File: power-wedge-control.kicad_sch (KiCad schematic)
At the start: 58 parts, among them J1 Conn_01x02, J2 Conn_01x03, J3 Conn_01x02, J4 Conn_01x03, J5 Conn_01x03, J6 Conn_01x06_Female, J7 Conn_01x04_Female, J8 Conn_01x03, J9 MicroSD_Hirose_DM3D-SF, Q1 MMBT3904L, Q2 DMP3099L, Q3 MMBT3904L, Q4 DMP3099L, Q5 MMBT3904L, Q6 MMBT3904L, U1 LM7805_TO220, U3 TLV70233DBV, U4 4050

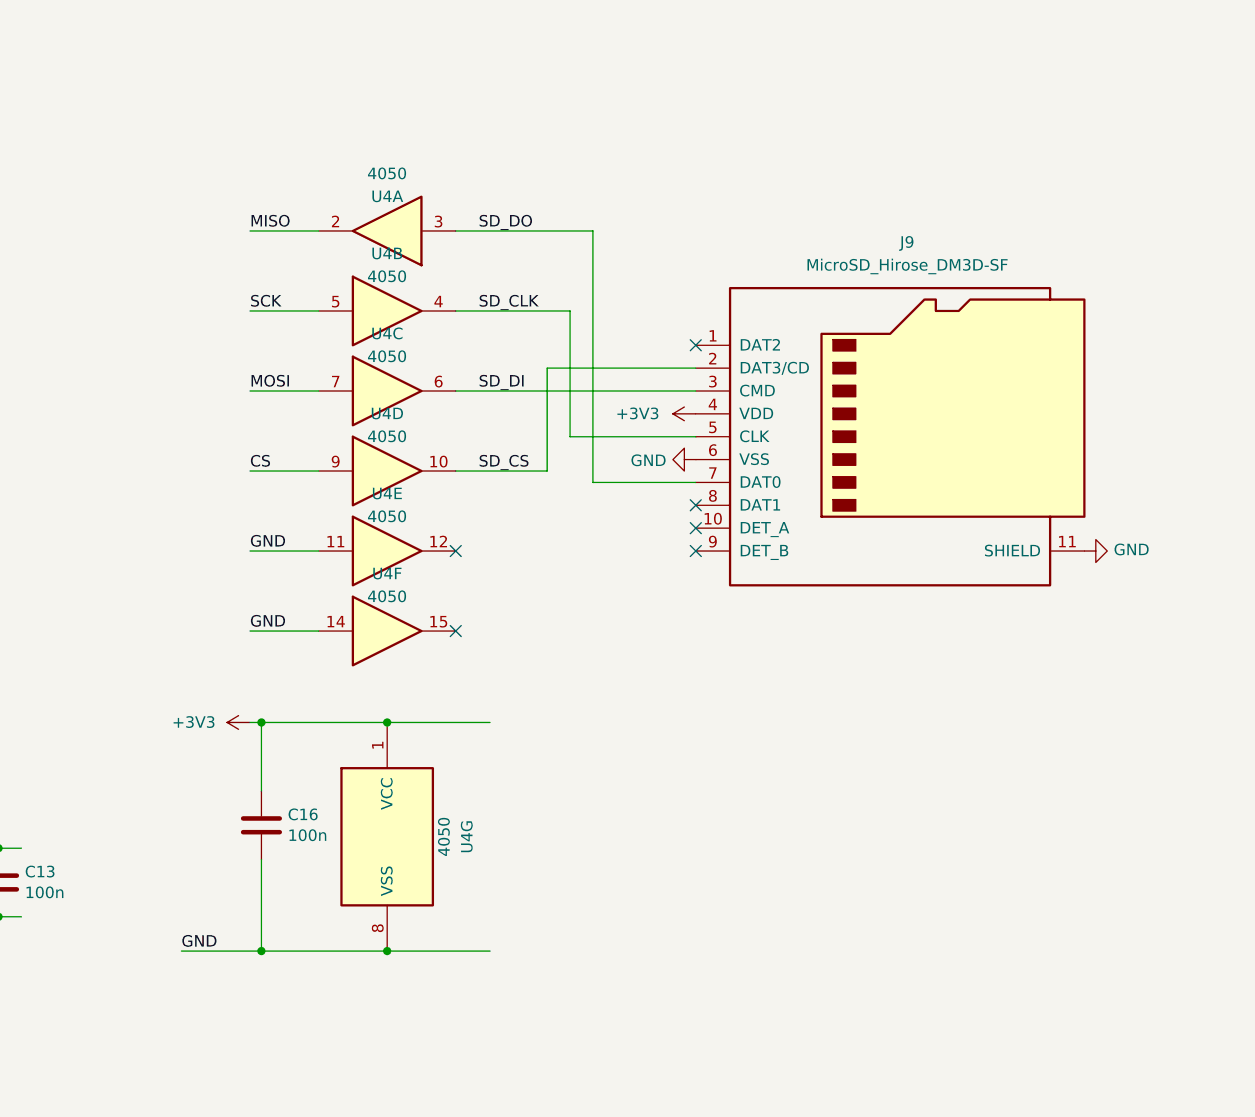
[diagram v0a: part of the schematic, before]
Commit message: Switch to NC7WZ17P6X buffers for level shifting to SD card.
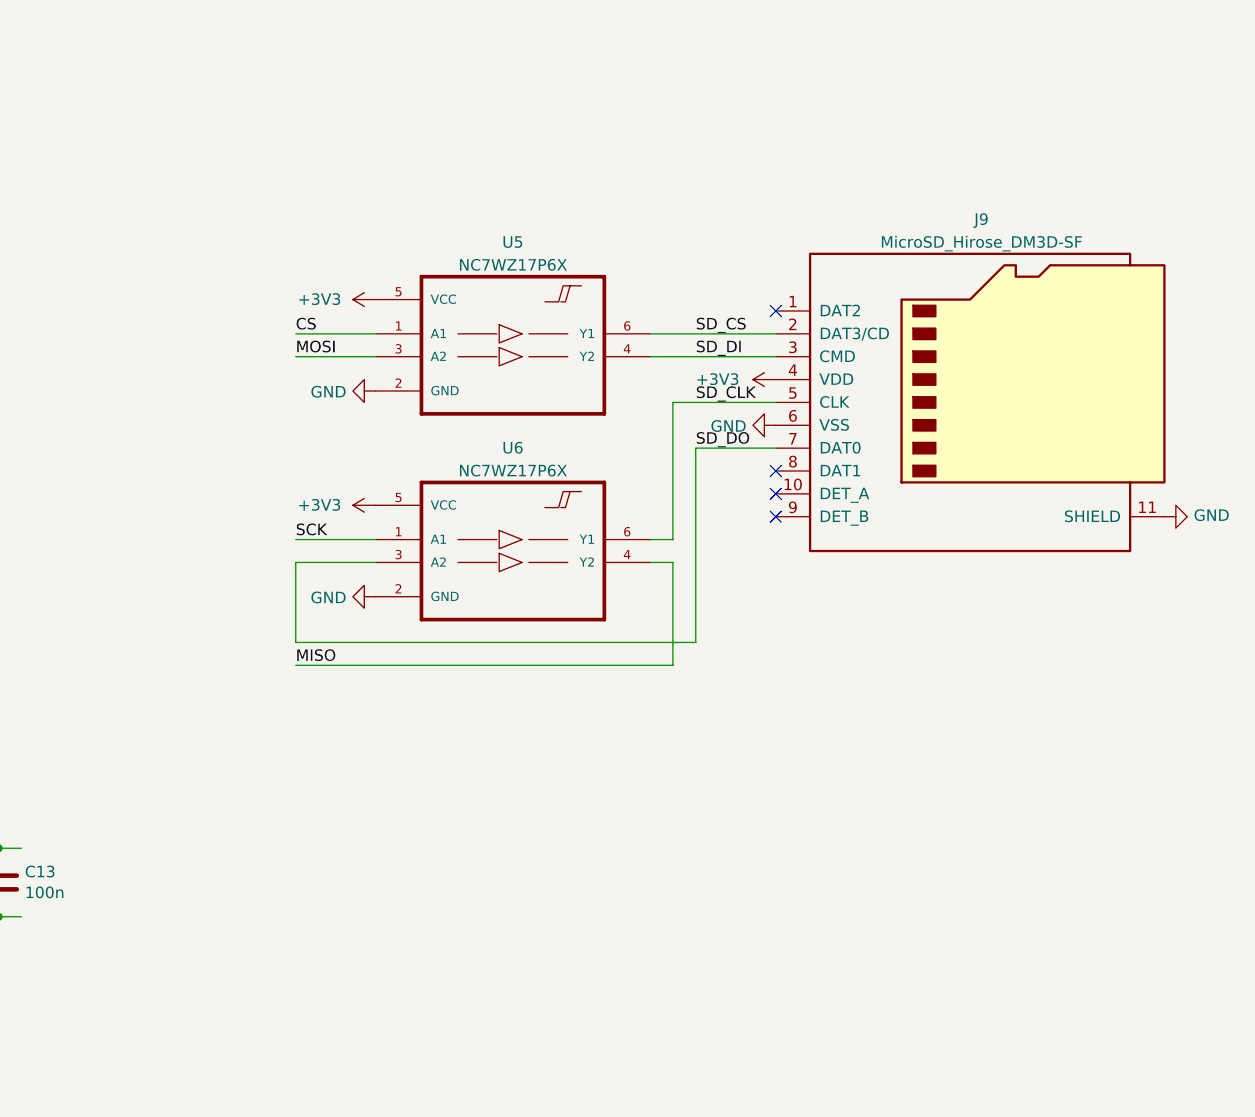
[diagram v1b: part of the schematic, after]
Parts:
- removed C16: 100n, Capacitor_SMD:C_0603_1608Metric, symbol Device:C
- removed U4: 4050, Package_SO:SOIC-16W_5.3x10.2mm_P1.27mm, symbol 4xxx:4050
- added U5, U6: NC7WZ17P6X, Package_TO_SOT_SMD:SOT-363_SC-70-6, symbol NC7WZ17P6X:NC7WZ17P6X
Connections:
- net +3V3: now also U5.5 (VCC), U6.5 (VCC)
- net CS: now also U5.1 (A1)
- net GND: now also U5.2 (GND), U6.2 (GND)
- net MISO: now also U6.4 (Y2)
- net MOSI: now also U5.3 (A2)
- net SCK: now also U6.1 (A1)
- net SD_CLK: now also U6.6 (Y1)
- net SD_CS: now also U5.6 (Y1)
- net SD_DI: now also U5.4 (Y2)
- net SD_DO: now also U6.3 (A2)
- no-connect marks 45 -> 43
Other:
- moved on the sheet: J9
